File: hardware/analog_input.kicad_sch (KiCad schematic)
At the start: 16 parts

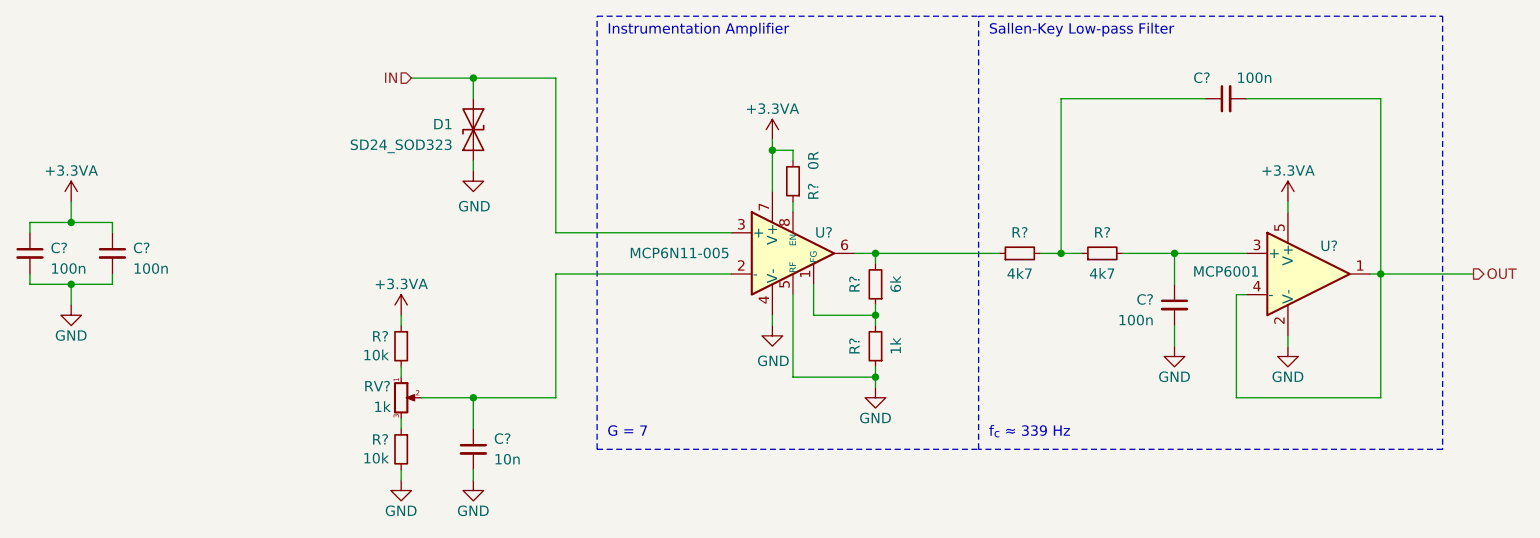
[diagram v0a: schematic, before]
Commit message: Add the Cube project
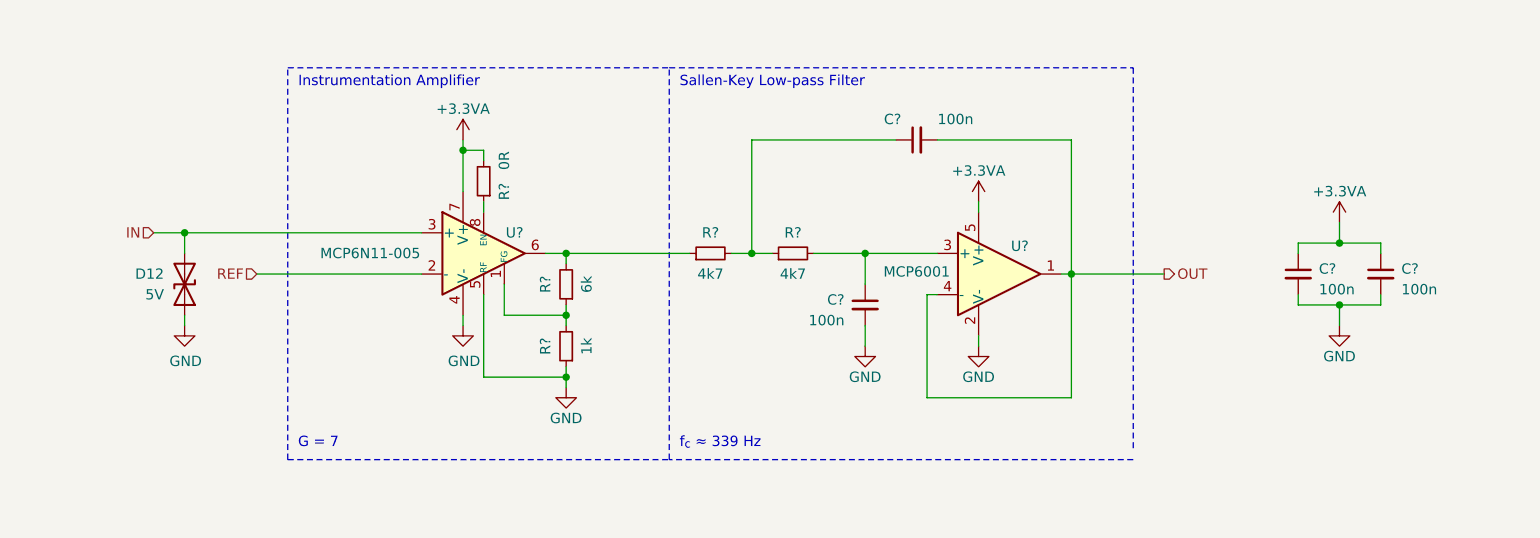
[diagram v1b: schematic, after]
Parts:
- removed C?: 10n, Capacitor_SMD:C_0603_1608Metric_Pad1.08x0.95mm_HandSolder, symbol Device:C_Small
- removed D1: SD24_SOD323, Diode_SMD:D_SOD-323_HandSoldering, symbol Diode:SD24_SOD323
- removed R? (x2): 10k, Resistor_SMD:R_0603_1608Metric_Pad0.98x0.95mm_HandSolder, symbol Device:R_Small
- removed RV?: 1k, Potentiometer_SMD:Potentiometer_Bourns_3214J_Horizontal, symbol Device:R_Potentiometer_Small
- added D12: 5V, symbol Device:D_TVS
- U?: footprint Package_DFN_QFN:TDFN-8-1EP_3x2mm_P0.5mm_EP1.3x1.4mm -> Package_DFN_QFN:TDFN-8-1EP_3x2mm_P0.5mm_EP1.80x1.65mm
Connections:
- net GND: now also D12.1 (A1)
- net IN: now also D12.2 (A2)
- net REF: now reaches U?.2 (-)
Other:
- company: (none) -> Author: I. Kajdan
- moved on the sheet: C?, R?, U?
